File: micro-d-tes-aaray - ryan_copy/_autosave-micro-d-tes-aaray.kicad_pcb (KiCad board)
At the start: 4 copper layers, 30 x 19.6 mm, 23 parts, among them J22 Conn_01x01_Socket, J23 Conn_01x01_Socket, J24 Conn_01x01_Socket, J25 Conn_01x01_Socket, J26 Conn_01x01_Socket, J27 Conn_01x01_Socket, J28 Conn_01x01_Socket, J29 Conn_01x01_Socket, J30 Conn_01x01_Socket, J31 Conn_01x01_Socket, J32 Conn_01x01_Socket, J33 Conn_01x01_Socket, J34 Conn_01x01_Socket, J35 Conn_01x01_Socket, J36 Conn_01x01_Socket, J37 Conn_01x01_Socket, J38 Conn_01x01_Socket, J39 Conn_01x01_Socket, J40 Conn_01x01_Socket, J41 Conn_01x01_Socket, J42 DB25_Plug

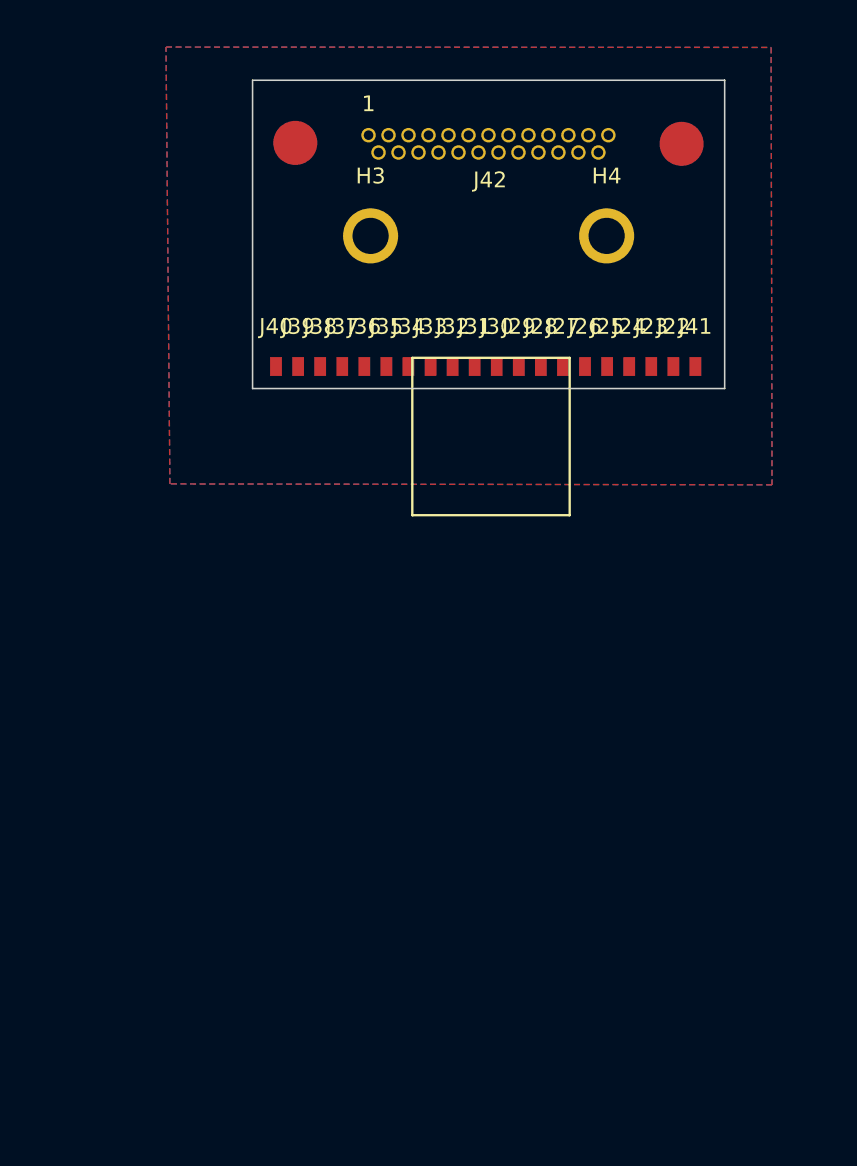
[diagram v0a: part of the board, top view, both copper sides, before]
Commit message: Update
finished old cad design
made new cad design
maybe finalized PCB layout
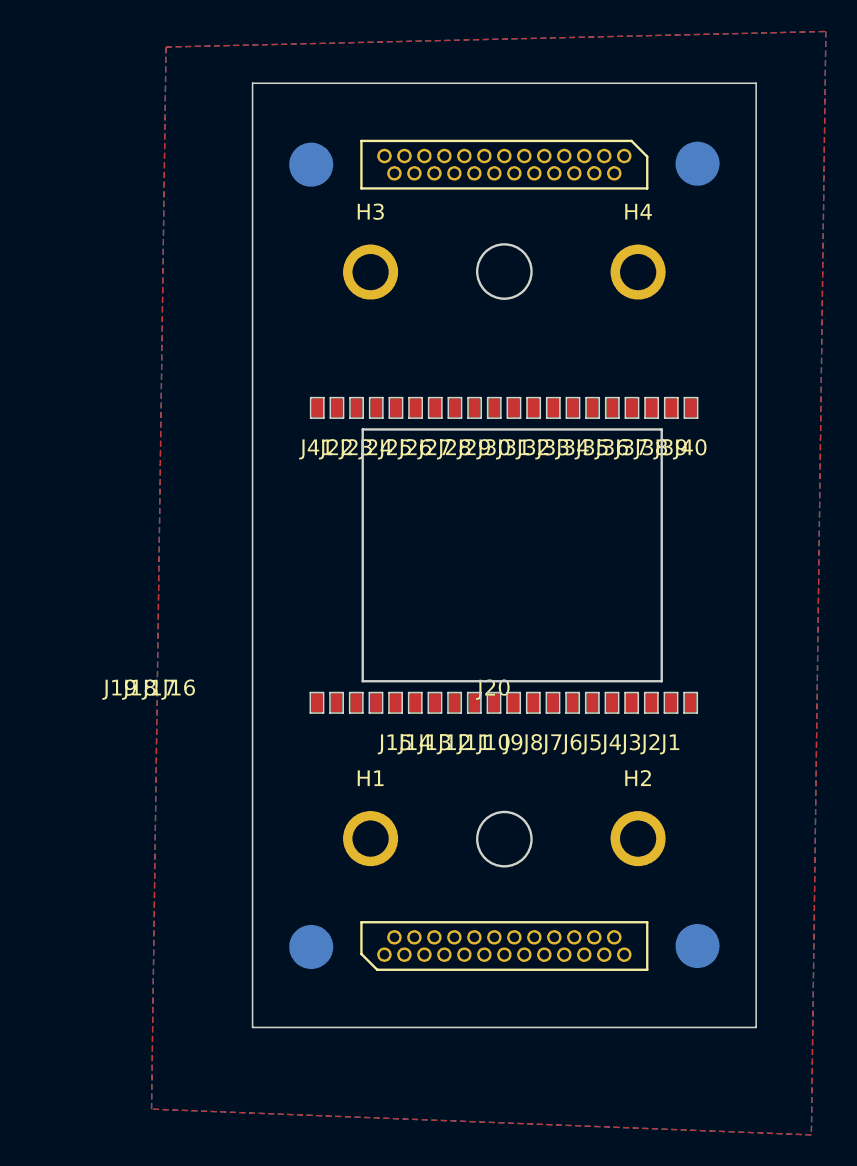
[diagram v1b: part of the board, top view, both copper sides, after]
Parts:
- added H1: MountingHole_Pad, 0_footprint_Library:MountingHole_3mm_2-56_DIN965_Pad, F.Cu at (7.50, 48.0)
- added H2: MountingHole_Pad, 0_footprint_Library:MountingHole_3mm_2-56_DIN965_Pad, F.Cu at (24.5, 48.0)
- added J1: Conn_01x01_Socket, 0_footprint_Library:SolderWirePad_1x01_SMD_0.5x0.5mm, F.Cu at (26.6, 39.4)
- added J10: Conn_01x01_Socket, 0_footprint_Library:SolderWirePad_1x01_SMD_0.5x0.5mm, F.Cu at (15.3, 39.4)
- added J11: Conn_01x01_Socket, 0_footprint_Library:SolderWirePad_1x01_SMD_0.5x0.5mm, F.Cu at (14.1, 39.4)
- added J12: Conn_01x01_Socket, 0_footprint_Library:SolderWirePad_1x01_SMD_0.5x0.5mm, F.Cu at (12.8, 39.4)
- added J13: Conn_01x01_Socket, 0_footprint_Library:SolderWirePad_1x01_SMD_0.5x0.5mm, F.Cu at (11.6, 39.4)
- added J14: Conn_01x01_Socket, 0_footprint_Library:SolderWirePad_1x01_SMD_0.5x0.5mm, F.Cu at (10.3, 39.4)
- added J15: Conn_01x01_Socket, 0_footprint_Library:SolderWirePad_1x01_SMD_0.5x0.5mm, F.Cu at (9.10, 39.4)
- added J16: Conn_01x01_Socket, 0_footprint_Library:SolderWirePad_1x01_SMD_0.5x0.5mm, F.Cu at (7.85, 39.4)
- added J17: Conn_01x01_Socket, 0_footprint_Library:SolderWirePad_1x01_SMD_0.5x0.5mm, F.Cu at (6.60, 39.4)
- added J18: Conn_01x01_Socket, 0_footprint_Library:SolderWirePad_1x01_SMD_0.5x0.5mm, F.Cu at (5.35, 39.4)
- added J19: Conn_01x01_Socket, 0_footprint_Library:SolderWirePad_1x01_SMD_0.5x0.5mm, F.Cu at (4.10, 39.4)
- added J2: Conn_01x01_Socket, 0_footprint_Library:SolderWirePad_1x01_SMD_0.5x0.5mm, F.Cu at (25.4, 39.4)
- added J20: Conn_01x01_Socket, 0_footprint_Library:SolderWirePad_1x01_SMD_0.5x0.5mm, F.Cu at (27.9, 39.4)
- added J21: DB25_Plug, 0_footprint_Library:Norcomp-380-025-113L001-microd_Updated, B.Cu at (16.0, 54.8)
- added J3: Conn_01x01_Socket, 0_footprint_Library:SolderWirePad_1x01_SMD_0.5x0.5mm, F.Cu at (24.1, 39.4)
- added J4: Conn_01x01_Socket, 0_footprint_Library:SolderWirePad_1x01_SMD_0.5x0.5mm, F.Cu at (22.9, 39.4)
- added J5: Conn_01x01_Socket, 0_footprint_Library:SolderWirePad_1x01_SMD_0.5x0.5mm, F.Cu at (21.6, 39.4)
- added J6: Conn_01x01_Socket, 0_footprint_Library:SolderWirePad_1x01_SMD_0.5x0.5mm, F.Cu at (20.4, 39.4)
- added J7: Conn_01x01_Socket, 0_footprint_Library:SolderWirePad_1x01_SMD_0.5x0.5mm, F.Cu at (19.1, 39.4)
- added J8: Conn_01x01_Socket, 0_footprint_Library:SolderWirePad_1x01_SMD_0.5x0.5mm, F.Cu at (17.9, 39.4)
- added J9: Conn_01x01_Socket, 0_footprint_Library:SolderWirePad_1x01_SMD_0.5x0.5mm, F.Cu at (16.6, 39.4)
- J42: moved to B.Cu
- moved J40 26.5 mm to (27.9, 20.6), turned to 180 degrees
- moved J41 24.2 mm to (4.11, 20.6), turned to 180 degrees
- moved J39 23.9 mm to (26.6, 20.6), turned to 180 degrees
- moved J22 21.5 mm to (5.36, 20.6), turned to 180 degrees
- moved J38 21.2 mm to (25.4, 20.6), turned to 180 degrees
- moved J23 18.9 mm to (6.61, 20.6), turned to 180 degrees
- moved J37 18.6 mm to (24.1, 20.6), turned to 180 degrees
- moved J24 16.3 mm to (7.86, 20.6), turned to 180 degrees
- moved J36 16.0 mm to (22.9, 20.6), turned to 180 degrees
- moved J25 13.7 mm to (9.11, 20.6), turned to 180 degrees
- moved J35 13.4 mm to (21.6, 20.6), turned to 180 degrees
- moved J26 11.1 mm to (10.4, 20.6), turned to 180 degrees
- moved J34 10.8 mm to (20.4, 20.6), turned to 180 degrees
- moved J27 8.53 mm to (11.6, 20.6), turned to 180 degrees
- moved J33 8.23 mm to (19.1, 20.6), turned to 180 degrees
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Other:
- board size 30 x 19.6 mm -> 32 x 60 mm
